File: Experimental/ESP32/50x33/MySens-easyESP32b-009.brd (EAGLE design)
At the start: 33 x 50 mm, 22 parts, among them U2 RFM69HCW, U3 ESP-WROOM-32

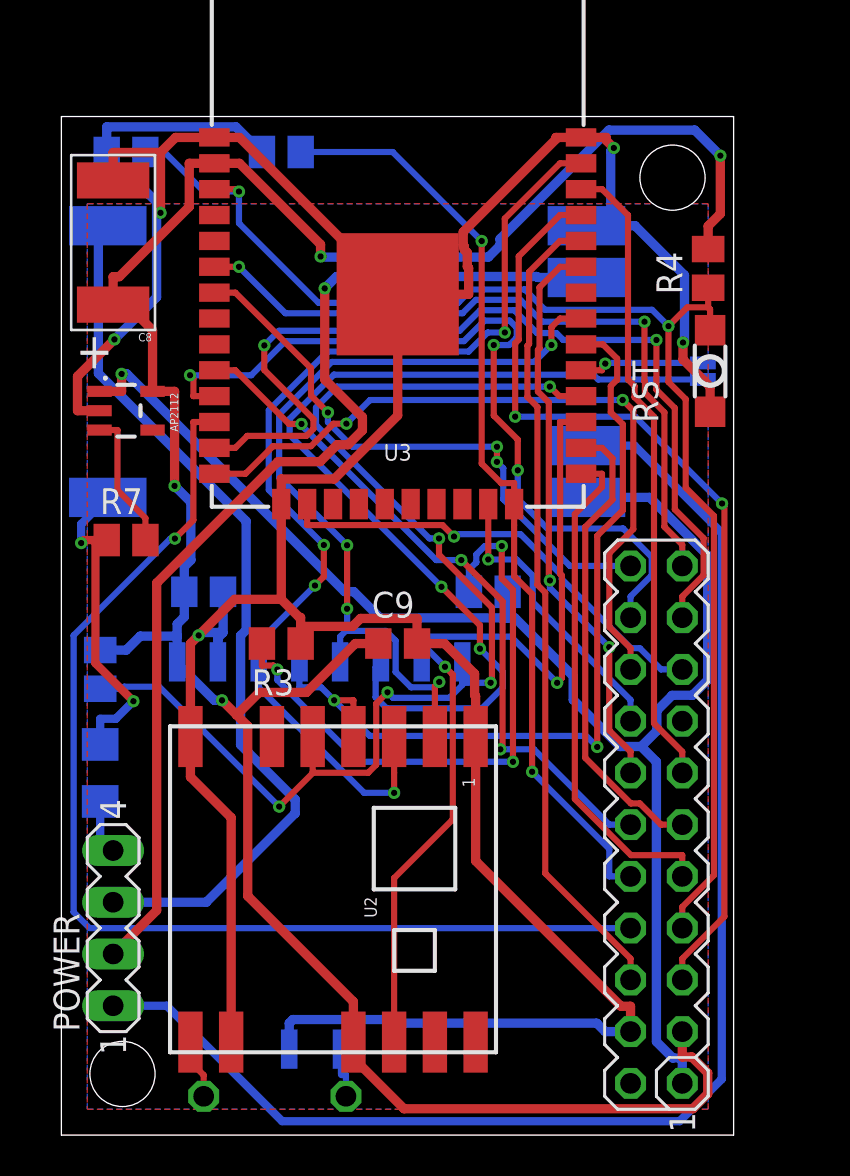
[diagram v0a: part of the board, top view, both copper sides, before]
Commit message: ESP32 AddOn
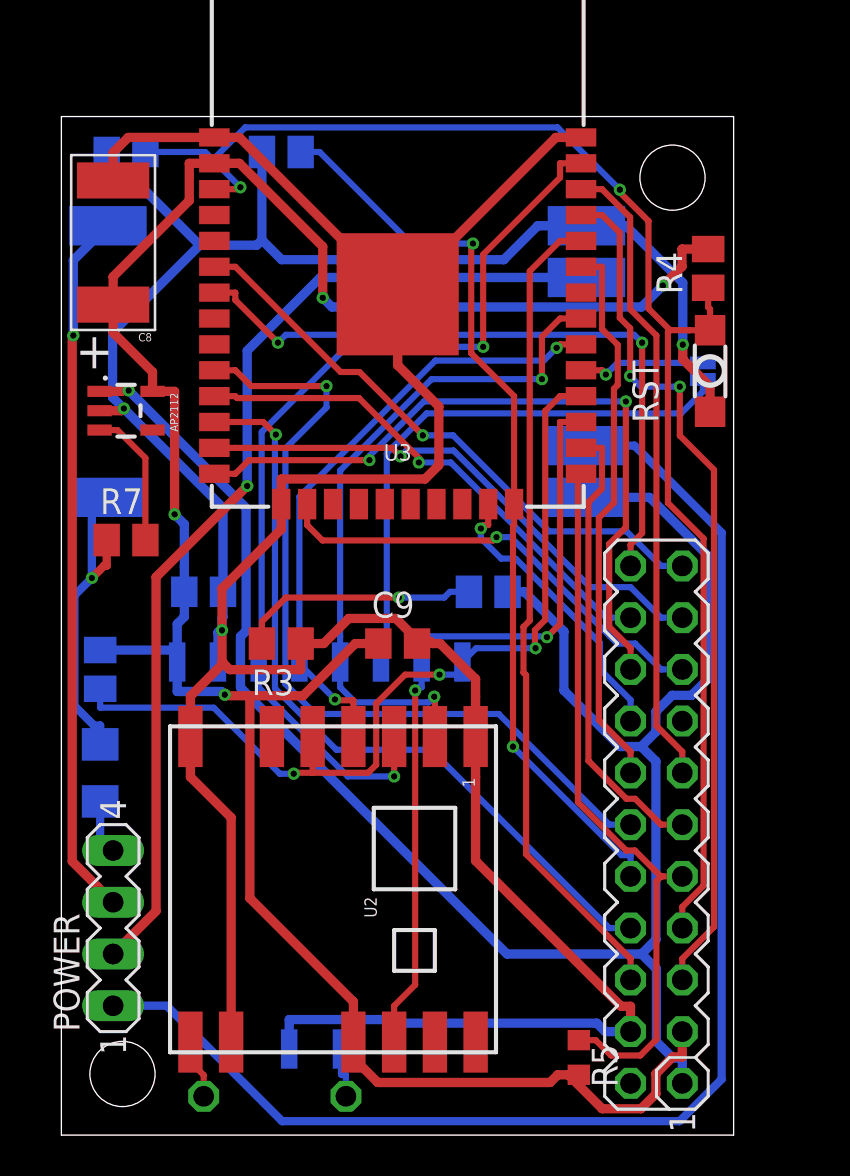
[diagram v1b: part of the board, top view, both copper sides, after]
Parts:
- added R5: 10k, rcl:R0603
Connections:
- net IO0: now also R5.1
- net VCC: now also R5.2
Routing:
- net MAYBE_IO5: track 47.5 -> 27.7 mm, vias 2 -> 0
- net IO14: track 45.9 -> 26.7 mm, vias 2 -> 1
- net GND: track 186.0 -> 205.1 mm, vias 5 -> 3
- net UREG: track 73.1 -> 91.7 mm
- net PB0: track 29.9 -> 11.8 mm, vias 3 -> 1
- net IO27: track 55.3 -> 38.1 mm
- net IO17: track 60.0 -> 44.0 mm, vias 5 -> 3
- net IO26: track 40.4 -> 25.1 mm, vias 3 -> 1
- net IO18: track 41.8 -> 30.3 mm
- net IO0: track 25.0 -> 35.4 mm
- net IN-: track 44.0 -> 34.8 mm, vias 0 -> 1
- net VCC: track 124.1 -> 116.8 mm
- net IO25: track 34.1 -> 41.1 mm, vias 3 -> 1
- net IO19: track 40.4 -> 33.8 mm, vias 4 -> 2
- net IO34: track 35.5 -> 29.1 mm, vias 2 -> 1
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- removed copper zone on layer 1, net GND
- removed copper zone on layer 16, net GND
